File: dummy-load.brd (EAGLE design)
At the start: 114.3 x 68.2 mm, 71 parts, among them T1 BU931P, T2 BU931P, T3 BU931P, T4 BU931P, T5 BU931P, T6 BU931P, T7 BU931P, T8 BU931P, U1 TLV272CD, U10 MCP4725A0T-E/CH, U2 TLV272CD, U3 TLV272CD, U4 TLV272CD, U5 TLV272CD, U6 TLV272CD, U7 TLV272CD, U8 TLV272CD, U9 MCP4725A0T-E/CH, X1 2524-

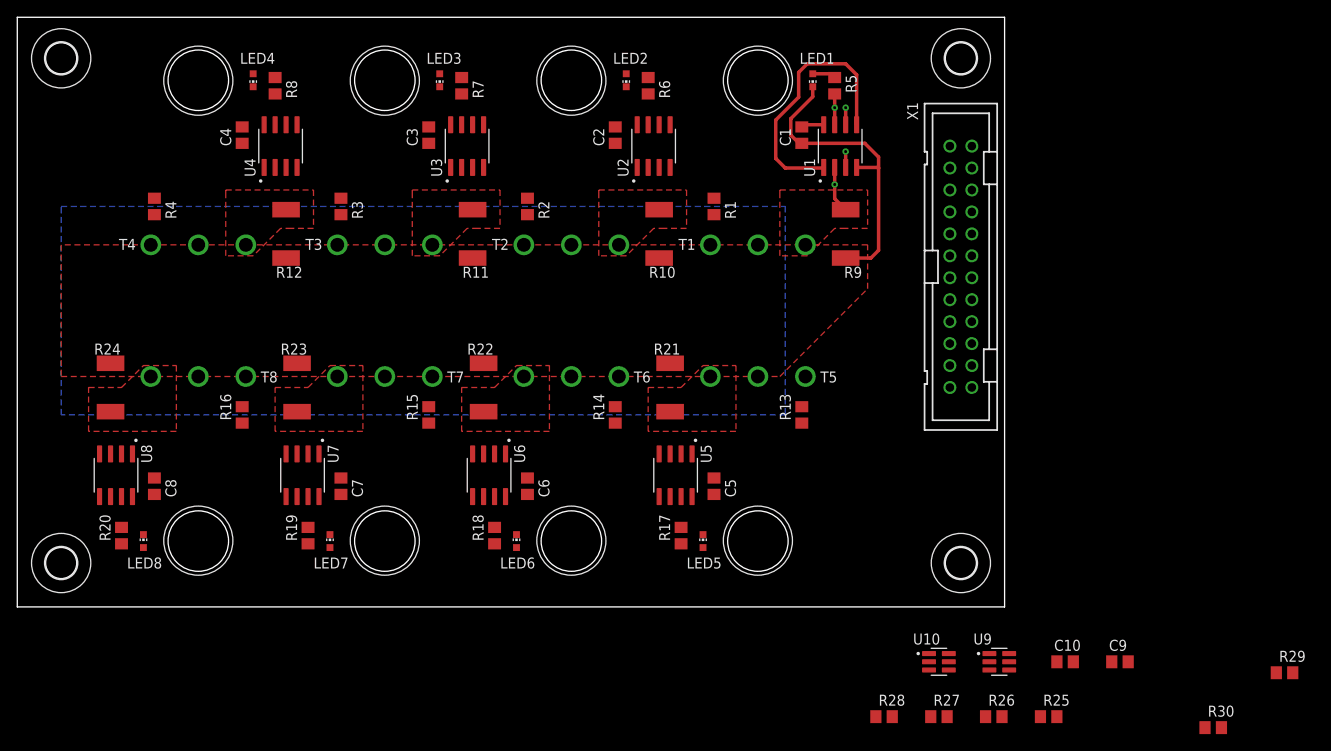
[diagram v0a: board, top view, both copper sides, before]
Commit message: PCB routing
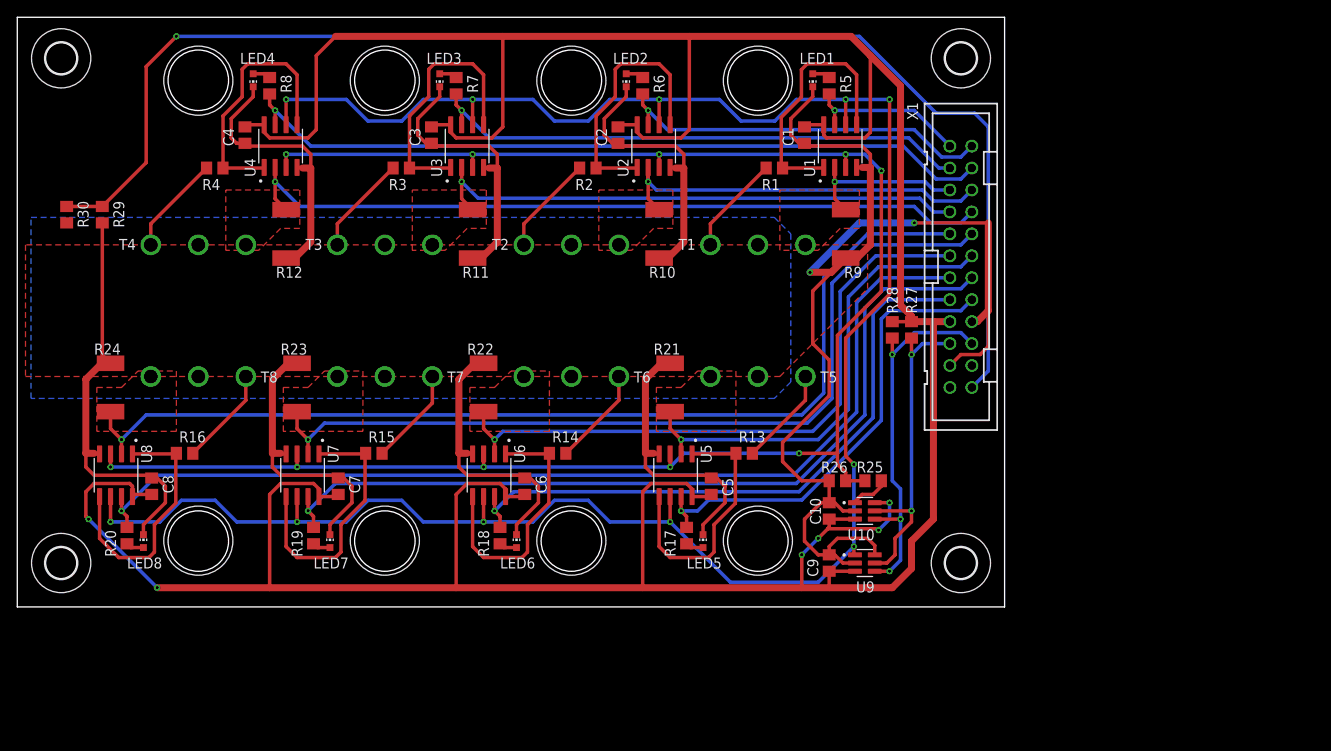
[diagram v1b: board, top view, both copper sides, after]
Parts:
- moved R29 146.8 mm to (9.84, 45.4), turned to 90 degrees
- moved R30 145.4 mm to (5.71, 45.4), turned to 270 degrees
- moved R27 44.9 mm to (103.5, 32.1), turned to 270 degrees
- moved R28 44.8 mm to (101.3, 32.1), turned to 270 degrees
- moved C9 35.5 mm to (94.0, 5.08), turned to 270 degrees
- moved R25 34.0 mm to (99.1, 14.6)
- moved R26 32.8 mm to (94.9, 14.6)
- moved C10 32.4 mm to (94.0, 11.1), turned to 270 degrees
- moved U10 19.5 mm to (98.1, 11.1)
- moved U9 19.3 mm to (98.1, 5.08)
- moved R2 8.28 mm to (66.0, 50.8), turned to 180 degrees
- moved R1 8.28 mm to (87.6, 50.8), turned to 180 degrees
- moved R3 8.28 mm to (44.5, 50.8), turned to 180 degrees
- moved R4 8.28 mm to (22.9, 50.8), turned to 180 degrees
- moved R13 8.01 mm to (84.1, 17.8), turned to 0 degrees
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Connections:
- net A1: now also X1.1; no longer X1.9
- net A2: now also X1.2; no longer X1.10
- net A3: now also X1.3; no longer X1.11
- net A4: now also X1.4; no longer X1.12
- net A5: now also X1.16; no longer X1.13
- net A6: now also X1.15; no longer X1.14
- net A7: now also X1.14; no longer X1.15
- net A8: now also X1.13; no longer X1.16
- net I1: now also X1.5; no longer X1.1
- net I2: now also X1.6; no longer X1.2
- net I3: now also X1.7; no longer X1.3
- net I4: now also X1.8; no longer X1.4
- net I5: now also X1.12; no longer X1.5
- net I6: now also X1.11; no longer X1.6
- net I7: now also X1.10; no longer X1.7
- net I8: now also X1.9; no longer X1.8
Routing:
- net +3V3: track 2.64 -> 415.3 mm, vias 0 -> 6
- net AGND: track 35.5 -> 386.3 mm, vias 0 -> 2
- net VACT: track 1.97 -> 251.6 mm, vias 1 -> 11
- net VSET: track 1.84 -> 207.2 mm, vias 1 -> 10
- net N$1: track 0.00 -> 156.6 mm, vias 0 -> 1
- net I8: track 0.00 -> 119.0 mm, vias 0 -> 1
- net A8: track 0.00 -> 118.3 mm, vias 0 -> 1
- net I7: track 0.00 -> 99.9 mm, vias 0 -> 1
- net A7: track 0.00 -> 99.1 mm, vias 0 -> 1
- net I4: track 0.00 -> 88.6 mm, vias 0 -> 1
- net A4: track 0.00 -> 88.3 mm, vias 0 -> 1
- net I6: track 0.00 -> 74.6 mm, vias 0 -> 1
- net A6: track 0.00 -> 73.7 mm, vias 0 -> 1
- net I3: track 0.00 -> 63.4 mm, vias 0 -> 1
- net A3: track 0.00 -> 63.1 mm, vias 0 -> 1
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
